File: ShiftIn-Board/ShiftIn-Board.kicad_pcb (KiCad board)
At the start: 2 copper layers, 30.5 x 20.3 mm, 5 parts, among them J1 Conn_01x06_Male, J2 Conn_01x06_Male, J3 Conn_01x08_Male, U1 74HC165_DIL16

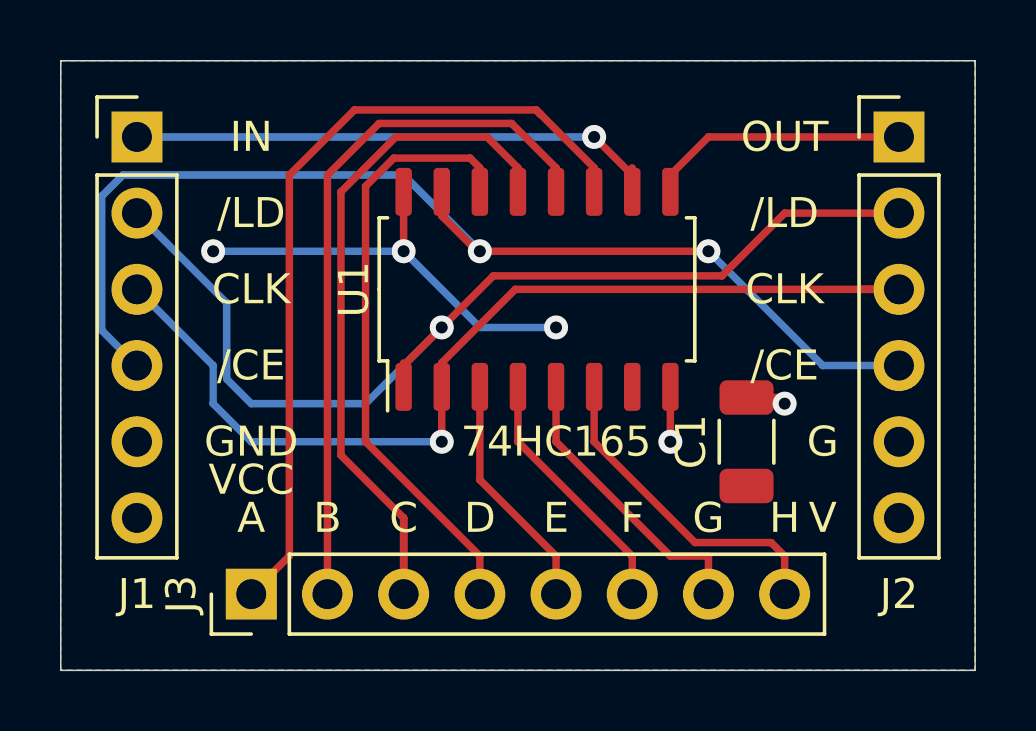
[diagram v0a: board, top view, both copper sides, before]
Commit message: Shiftin-Board v0.2
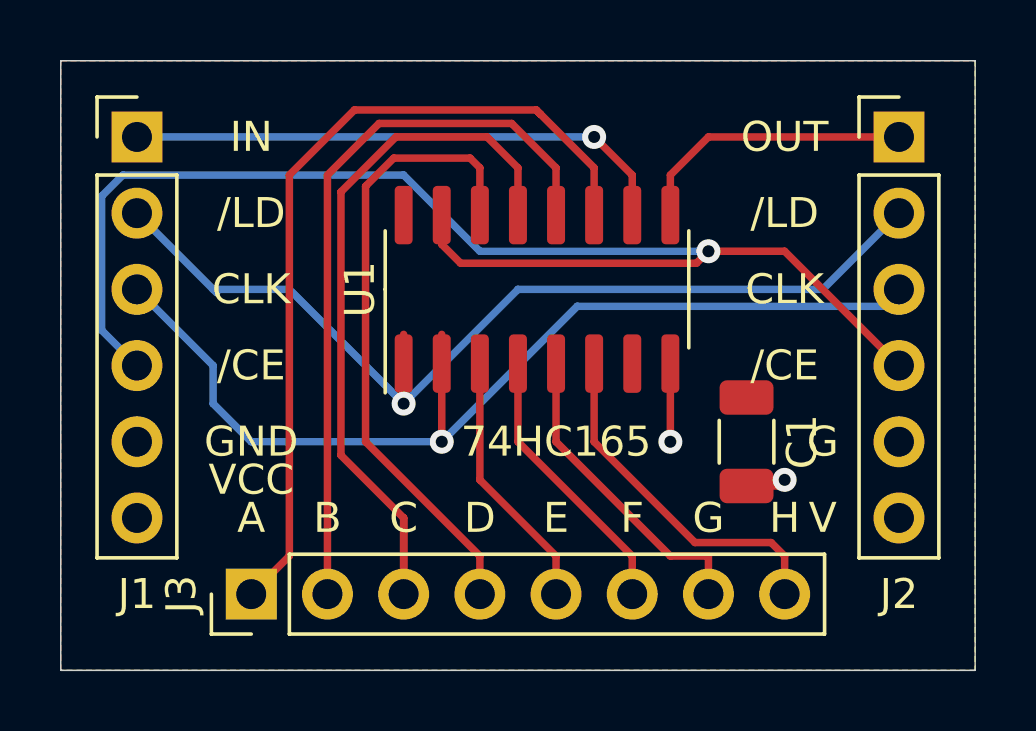
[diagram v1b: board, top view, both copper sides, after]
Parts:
- U1: footprint Package_SO:SOIC-16_4.55x10.3mm_P1.27mm -> Package_SO:SOIC-16_3.9x9.9mm_P1.27mm
- turned C1 to 270 degrees
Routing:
- net VCC: track 15.2 -> 0.71 mm, vias 3 -> 0
- net Net-(J1-Pad4): track 38.2 -> 46.7 mm, vias 2 -> 1
- net Net-(J1-Pad2): track 35.5 -> 34.6 mm
- net Net-(J1-Pad1): track 18.4 -> 17.6 mm
- net Net-(J1-Pad3): track 33.2 -> 34.0 mm
